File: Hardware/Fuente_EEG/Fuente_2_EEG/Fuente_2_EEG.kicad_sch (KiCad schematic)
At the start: 24 parts, among them J1 BJ_V1, J2 BJ_V2, J3 TB_V1, J4 TB_V2, J5 VOUT, J6 Moutning Hole

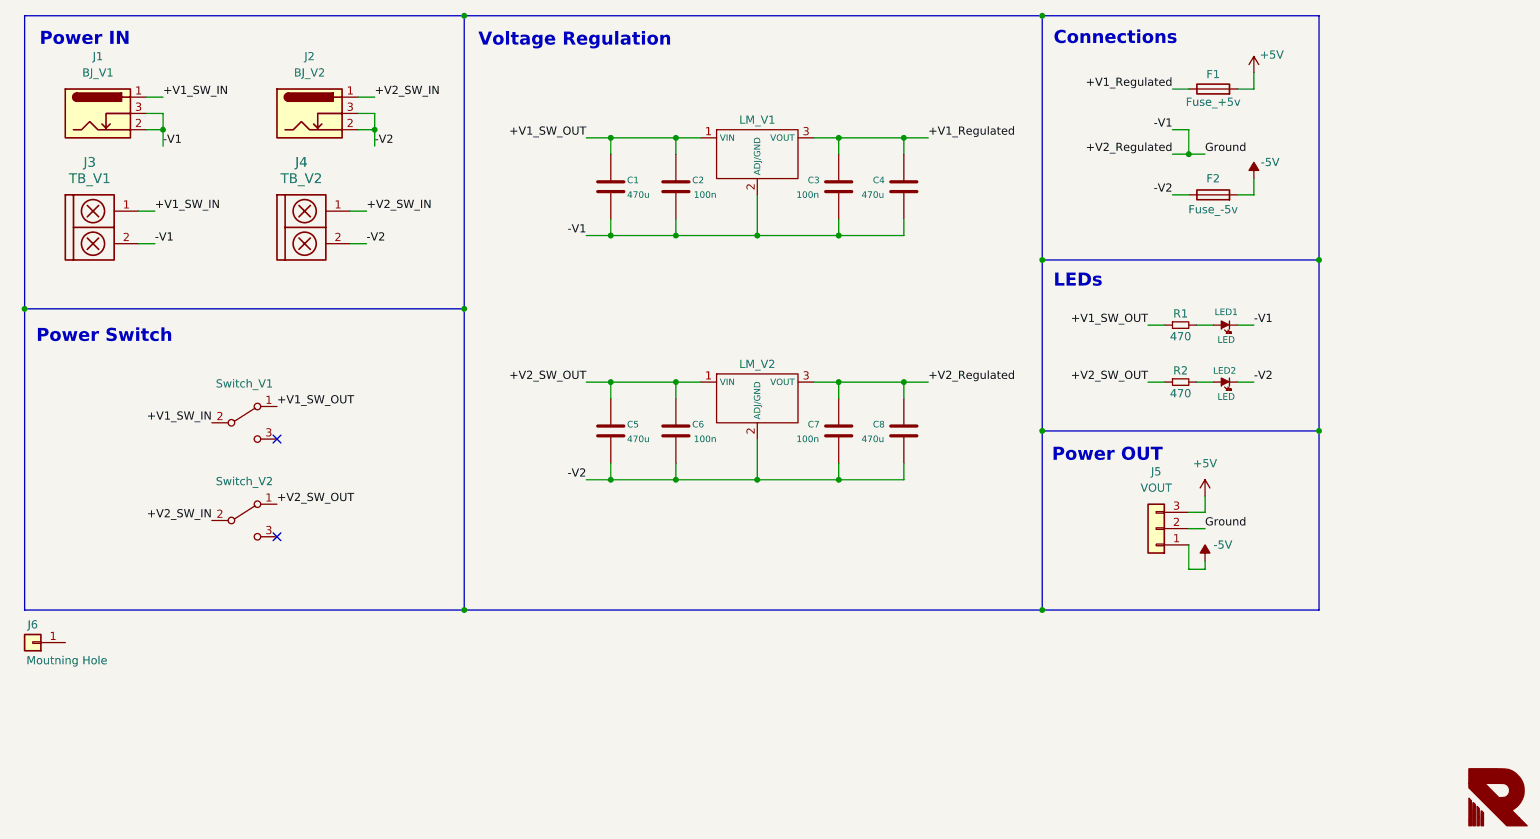
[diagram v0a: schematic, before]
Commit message: Fuente Update
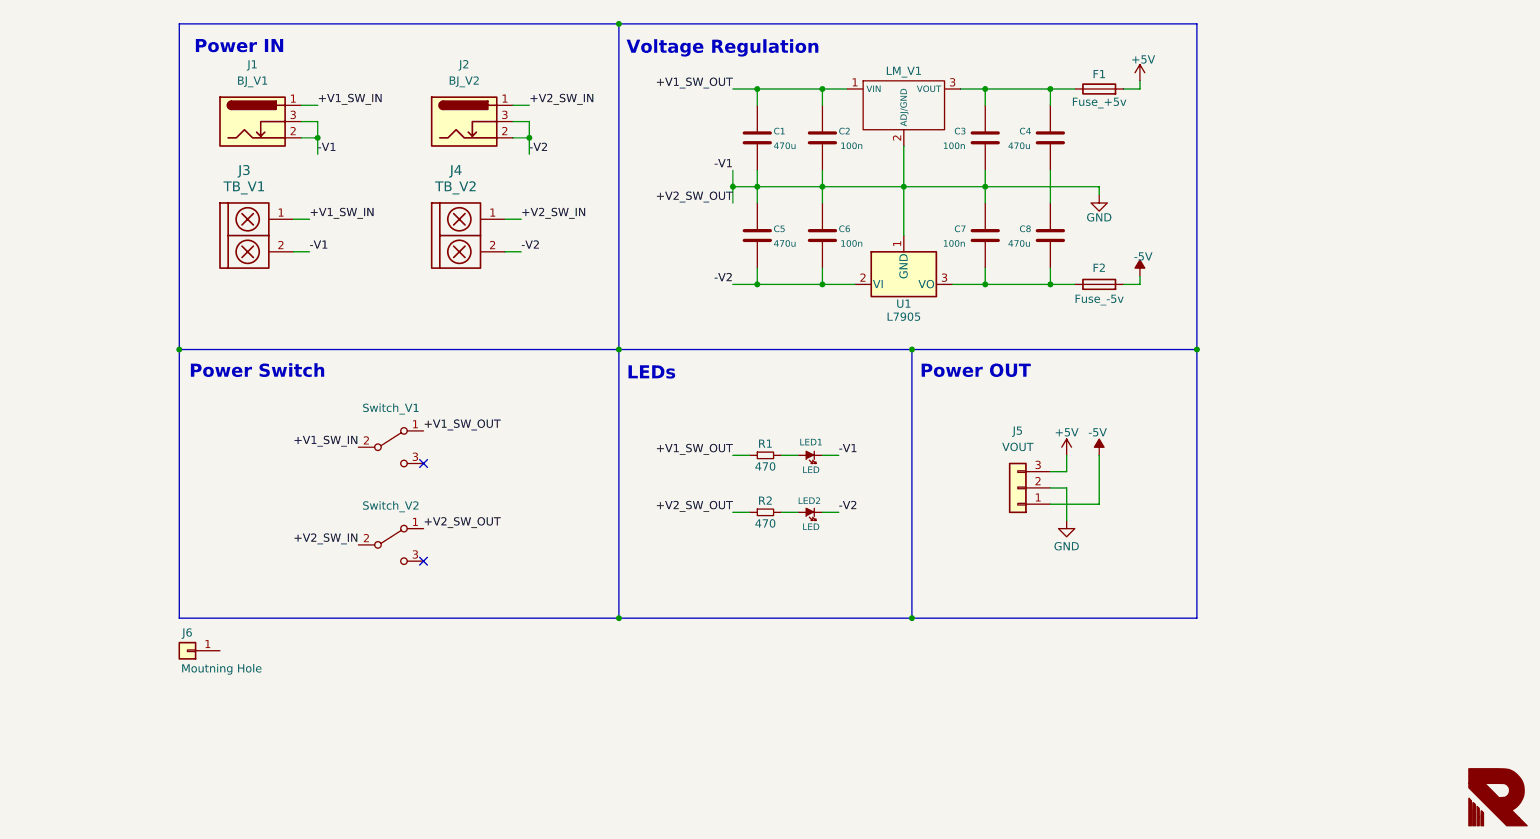
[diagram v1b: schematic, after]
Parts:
- removed LM_V2: ~, EESTN5:TO-220, symbol Logo_Romano:LM7805
- added U1: L7905, EESTN5:TO-220, symbol Regulator_Linear:L7905
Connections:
- net +V2_SW_OUT is gone; now on net GND: C5.1, C6.1, R2.1, Switch_V2.1 (A)
- net -V2: now also U1.2 (VI); no longer C7.2, C8.2, F2.1
- net +V1_Regulated: no longer names the net of C3.1, C4.1, F1.1, LM_V1.3 (VOUT)
- net +V2_Regulated renamed GND
- net GND: now also U1.1 (GND); no longer C4.2, C8.1
- new net: C7.2, C8.2, F2.1, U1.3 (VO)
- new net: C4.2, C8.1
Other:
- note removed: "Connections"
- moved on the sheet: C1, C2, C3, C4, C5, C6, C7, C8, F1, F2, J1, J2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
